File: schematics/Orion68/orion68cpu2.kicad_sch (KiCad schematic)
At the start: 66 parts, among them J1 Euro96pin, J2 clock, J3 clock1, Q1 2N3904, Q2 2N3904, Q3 2N3904, SW2 sw_reset, U0 MC68000FN, U08 GAL16V8, U09 GAL20V8, U1 74LS245, U10 SST39SF010, U11 74HC74, U12 74LS393, U13 74HC138, U14 74HC138, U15 74HC138, U17 74LS139, U2 74LS245, U3 74LS541, U4 74LS541, U5 74LS541, U6 74LS541, U7 74LS148, U9 SST39SF010

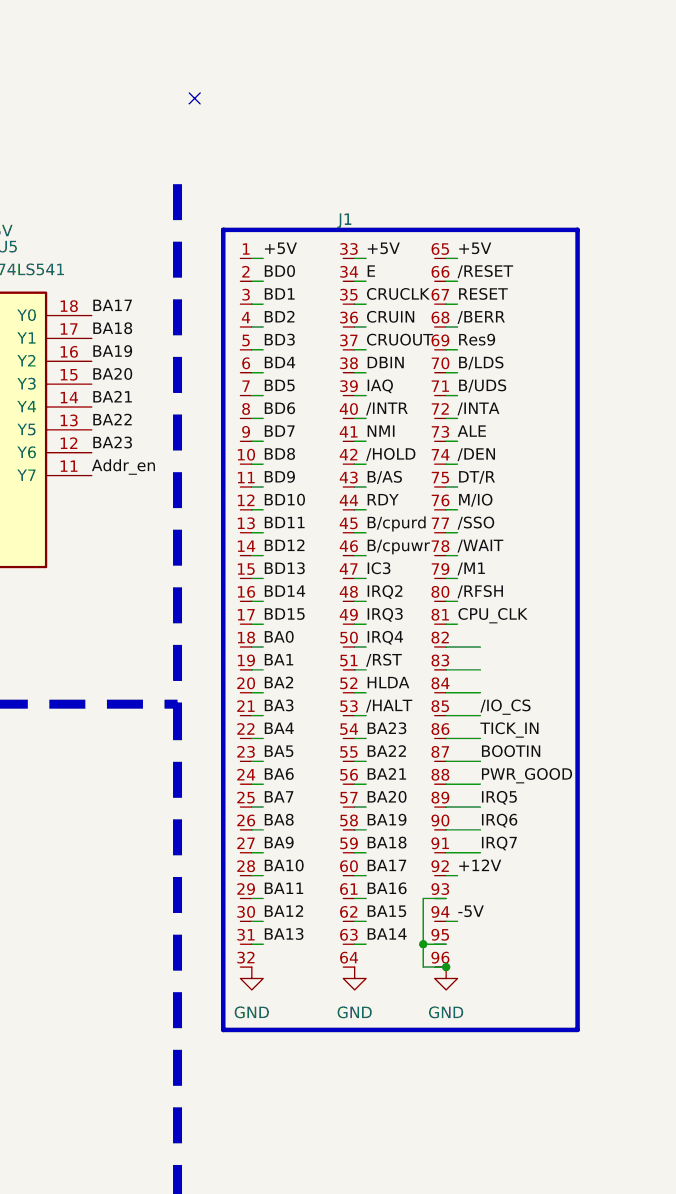
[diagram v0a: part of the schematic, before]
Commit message: update
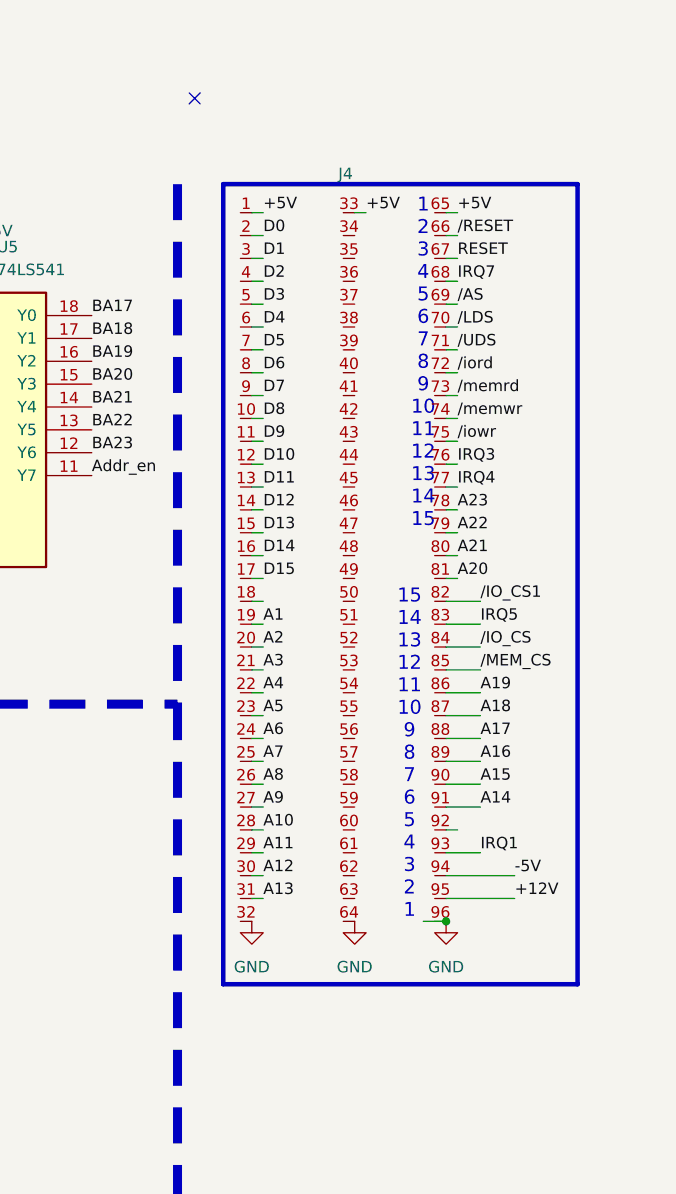
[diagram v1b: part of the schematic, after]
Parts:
- removed J1: Euro96pin, ConnPdSilva:conn_euro96, symbol ConnPdSilva:ConnEuro96
- added J4: Euro96pin, ConnPdSilva:conn_euro96, symbol ConnPdSilva:ConnEuro96
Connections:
- net +12V: now also J4.95
- net +5V: now also J4.1, J4.33, J4.65
- net -5V: now also J4.94
- net A1: now also J4.19
- net A10: now also J4.28
- net A11: now also J4.29
- net A12: now also J4.30
- net A13: now also J4.31
- net A14: now also J4.91
- net A15: now also J4.90
- net A16: now also J4.89
- net A17: now also J4.88
- net A18: now also J4.87
- net A19: now also J4.86
- net A2: now also J4.20
- net A20: now also J4.81
- net A21: now also J4.80
- net A22: now also J4.79
- net A23: now also J4.78
- net A3: now also J4.21
- net A4: now also J4.22
- net A5: now also J4.23
- net A6: now also J4.24
- net A7: now also J4.25
- net A8: now also J4.26
- net A9: now also J4.27
- net D0: now also J4.2
- net D1: now also J4.3
- net D10: now also J4.12
- net D11: now also J4.13
- net D12: now also J4.14
- net D13: now also J4.15
- net D14: now also J4.16
- net D15: now also J4.17
- net D2: now also J4.4
- net D3: now also J4.5
- net D4: now also J4.6
- net D5: now also J4.7
- net D6: now also J4.8
- net D7: now also J4.9
- net D8: now also J4.10
- net D9: now also J4.11
- net GND: now also J4.32, J4.64, J4.96
- net IRQ3: now also J4.76
- net IRQ4: now also J4.77
- net IRQ5: now also J4.83
- net IRQ7: now also J4.68
- net RESET: now also J4.67
- net /AS: now also J4.69
- net /IO_CS: now also J4.84
- net /LDS: now also J4.70
- net /RESET: now also J4.66
- net /UDS: now also J4.71
- new net IRQ1: J4.93
- new net /IO_CS1: J4.82
- new net /MEM_CS: J4.85
- new net /iord: J4.72
- new net /iowr: J4.75
- new net /memrd: J4.73
- new net /memwr: J4.74
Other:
- note added: "1 2 3 4 5 6 7 8 9 10 11 12 13 14 15"
- note added: "15 14 13 12 11 10 9 8 7 6 5 4 3 2 1"
